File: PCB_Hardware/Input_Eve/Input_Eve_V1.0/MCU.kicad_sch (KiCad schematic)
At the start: 15 parts, among them J1 Conn_ARM_JTAG_SWD_10, U1 STM32H743VITx

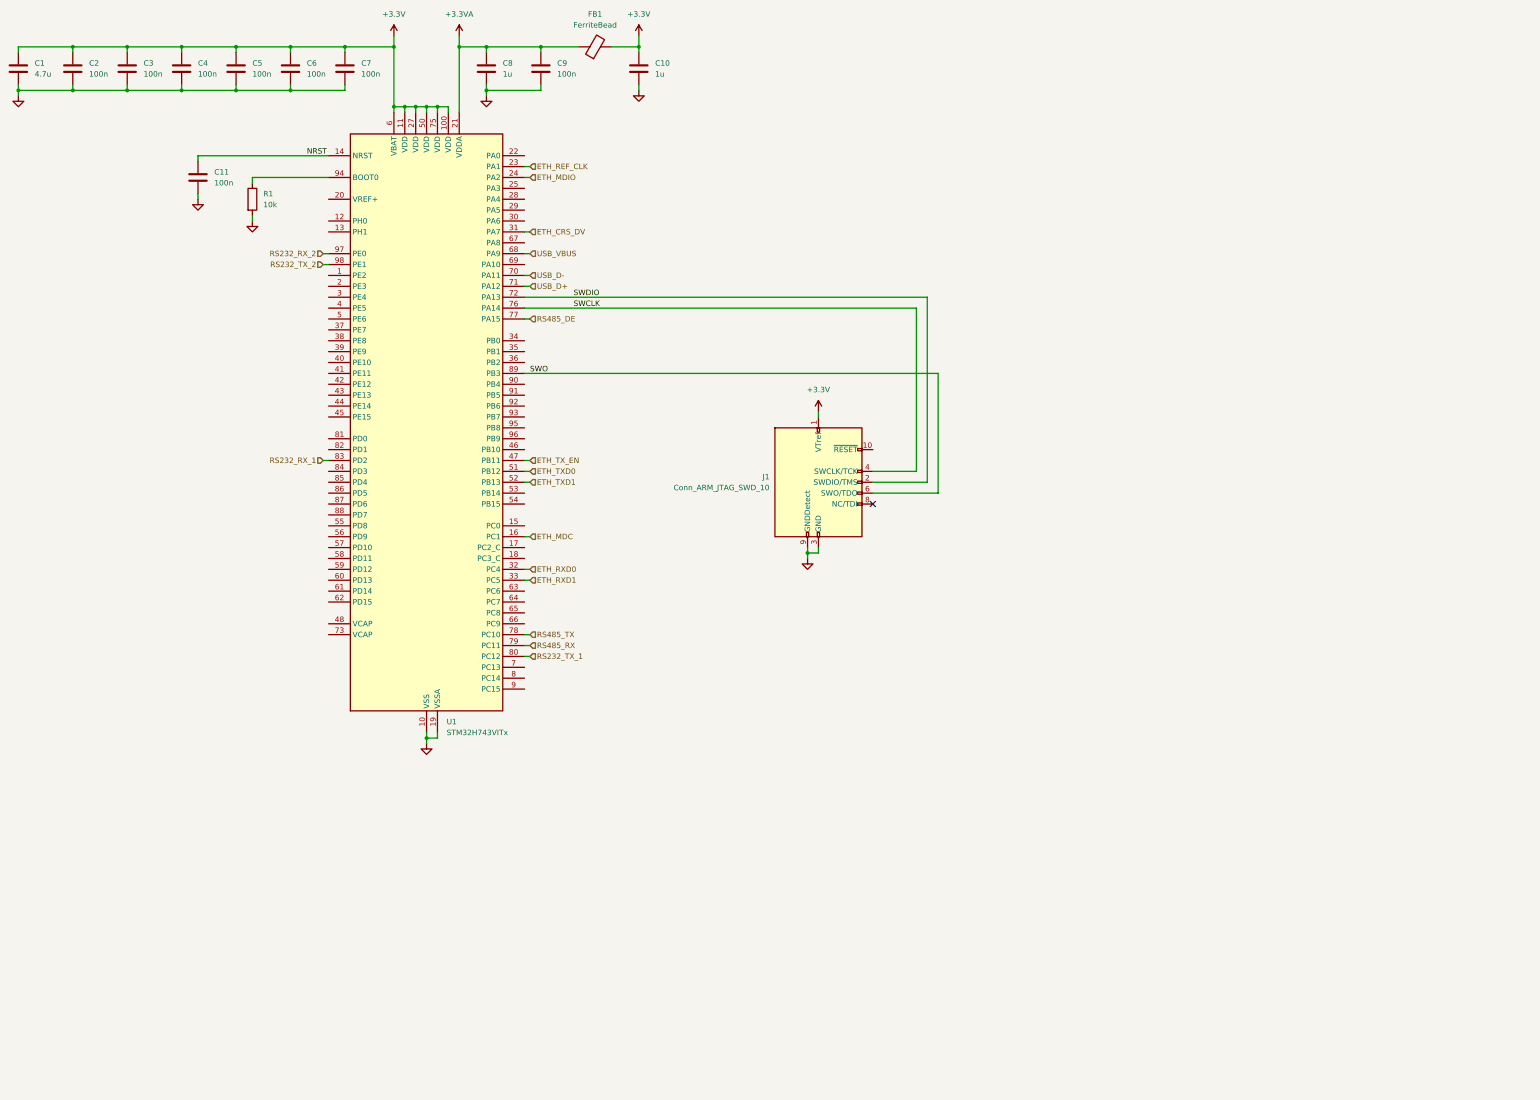
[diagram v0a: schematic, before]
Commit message: Update w new boards/firmware
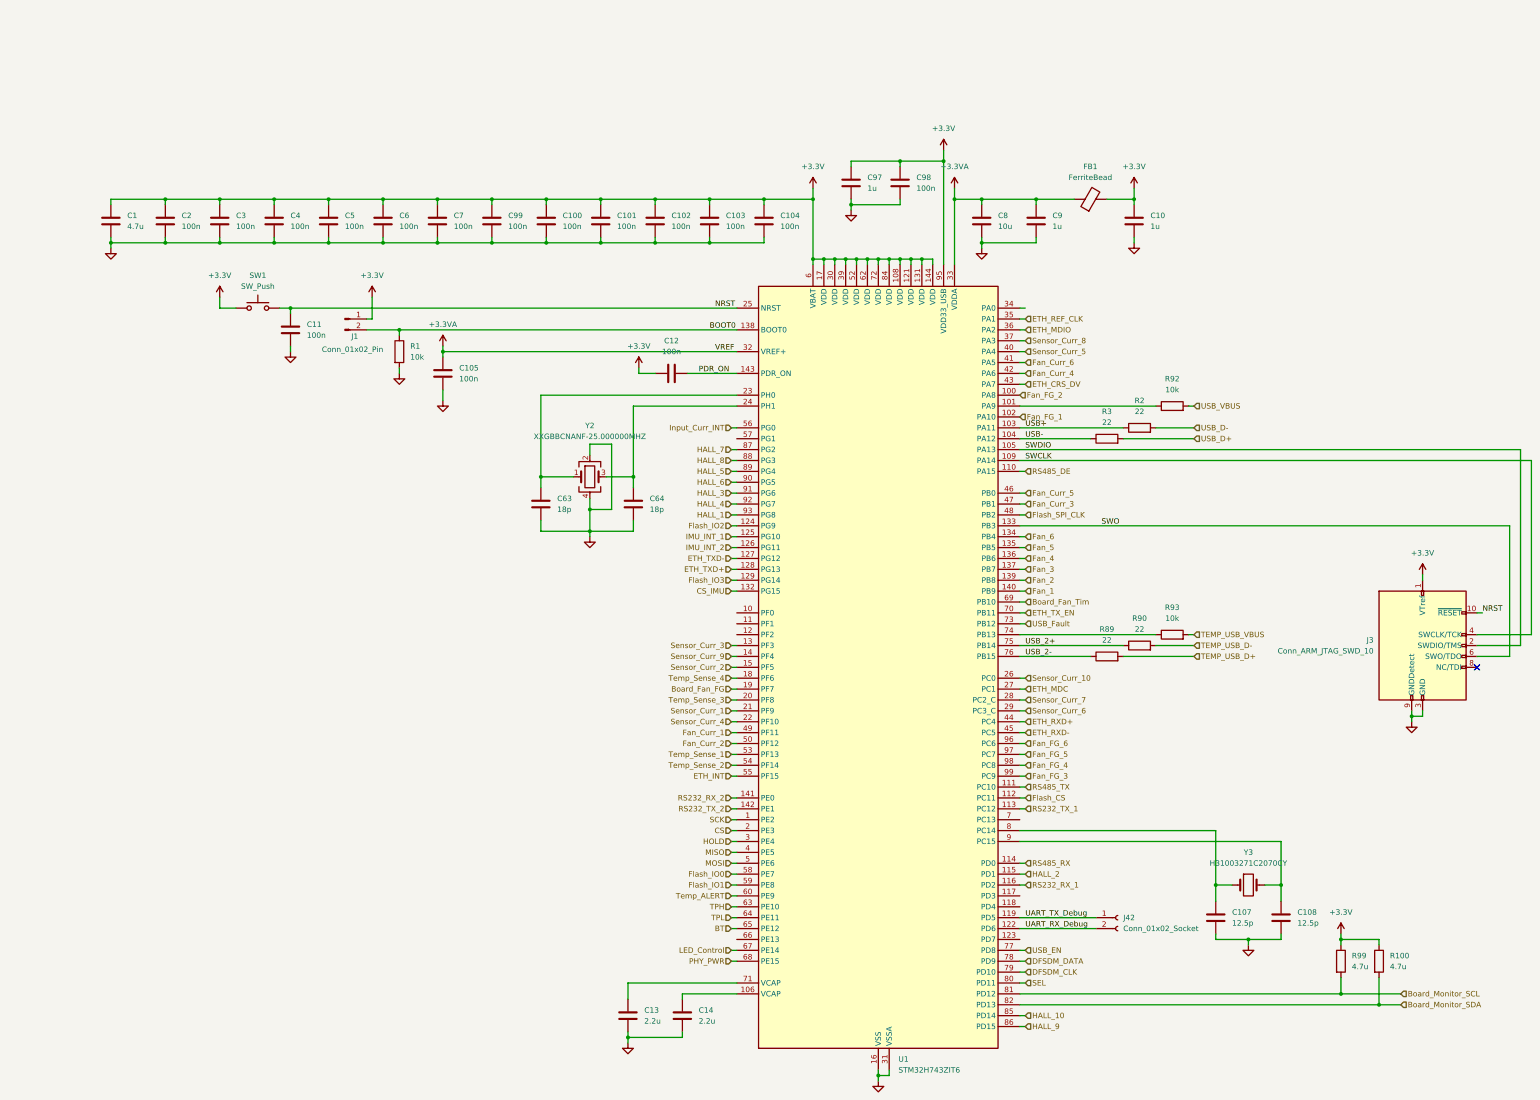
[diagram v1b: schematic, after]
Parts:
- removed U1: STM32H743VITx, Package_QFP:LQFP-100_14x14mm_P0.5mm, symbol MCU_ST_STM32H7:STM32H743VITx
- added C100, C101, C102, C103, C104, C105, C12, C98, C99: 100n, Capacitor_SMD:C_0402_1005Metric, symbol Device:C
- added C107, C108: 12.5p, Capacitor_SMD:C_0402_1005Metric, symbol Device:C
- added C13, C14: 2.2u, Capacitor_SMD:C_0402_1005Metric, symbol Device:C
- added C63, C64: 18p, Capacitor_SMD:C_0402_1005Metric, symbol Device:C
- added C97: 1u, Capacitor_SMD:C_0402_1005Metric, symbol Device:C
- added J1: Conn_01x02_Pin, Connector_PinHeader_2.54mm:PinHeader_1x02_P2.54mm_Vertical, symbol Connector:Conn_01x02_Pin
- added J42: Conn_01x02_Socket, Connector_JST:JST_PH_B2B-PH-K_1x02_P2.00mm_Vertical, symbol Connector:Conn_01x02_Socket
- added R100, R99: 4.7u, Resistor_SMD:R_0402_1005Metric, symbol Device:R
- added R2, R3, R89, R90: 22, Resistor_SMD:R_0402_1005Metric, symbol Device:R
- added R92, R93: 10k, Resistor_SMD:R_0402_1005Metric, symbol Device:R
- added SW1: SW_Push, Tutor_Common_Parts:TSB008A2518A, symbol Switch:SW_Push
- added U1: STM32H743ZIT6, Package_QFP:LQFP-144_20x20mm_P0.5mm, symbol MCU_ST_STM32H7:STM32H743ZITx
- added Y2: XXGBBCNANF-25.000000MHZ, Crystal:Crystal_SMD_3225-4Pin_3.2x2.5mm, symbol Device:Crystal_GND24
- added Y3: H31003271C2070CY, Crystal:Crystal_SMD_3215-2Pin_3.2x1.5mm, symbol Device:Crystal
- C1: footprint (none) -> Capacitor_SMD:C_0603_1608Metric
- C10, C11, C2, C3, C4, C5, C6, C7: footprint (none) -> Capacitor_SMD:C_0402_1005Metric
- C8: renamed from C9; value 100n -> 10u; footprint (none) -> Capacitor_SMD:C_0402_1005Metric
- C9: renamed from C8; footprint (none) -> Capacitor_SMD:C_0402_1005Metric
- FB1: footprint (none) -> Inductor_SMD:L_0603_1608Metric
- J3: renamed from J1; footprint (none) -> Connector_PinHeader_1.27mm:PinHeader_2x05_P1.27mm_Vertical_SMD
- R1: footprint (none) -> Resistor_SMD:R_0402_1005Metric
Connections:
- net +3.3V: now also C100.1, C101.1, C102.1, C103.1, C104.1, C12.1, C97.1, C98.1, C99.1, J1.1 (Pin_1), R100.1, R99.1, SW1.1, U1.108 (VDD), U1.121 (VDD), U1.131 (VDD), U1.144 (VDD), U1.17 (VDD), U1.30 (VDD), U1.39 (VDD), U1.52 (VDD), U1.6 (VBAT), U1.62 (VDD), U1.72 (VDD), U1.84 (VDD), U1.95 (VDD33_USB)
- net +3.3VA: now also C105.2, U1.32 (VREF+), U1.33 (VDDA)
- net ETH_CRS_DV: now also U1.43 (PA7)
- net ETH_MDC: now also U1.27 (PC1)
- net ETH_MDIO: now also U1.36 (PA2)
- net ETH_REF_CLK: now also U1.35 (PA1)
- net ETH_TX_EN: now also U1.70 (PB11)
- net GND: now also C100.2, C101.2, C102.2, C103.2, C104.2, C105.1, C107.2, C108.2, C13.2, C14.2, C63.2, C64.2, C97.2, C98.2, C99.2, U1.107 (VSS), U1.120 (VSS), U1.130 (VSS), U1.16 (VSS), U1.31 (VSSA), U1.38 (VSS), U1.51 (VSS), U1.61 (VSS), U1.83 (VSS), U1.94 (VSS), Y2.2, Y2.4
- net NRST: now also J3.10 (~{RESET}), SW1.2, U1.25 (NRST)
- net RS232_RX_1: now also U1.116 (PD2)
- net RS232_RX_2: now also U1.141 (PE0)
- net RS232_TX_1: now also U1.113 (PC12)
- net RS232_TX_2: now also U1.142 (PE1)
- net RS485_DE: now also U1.110 (PA15)
- net RS485_RX: now also U1.114 (PD0)
- net RS485_TX: now also U1.111 (PC10)
- net SWCLK: now also U1.109 (PA14)
- net SWDIO: now also U1.105 (PA13)
- net SWO: now also U1.133 (PB3)
- net USB_D+: now also R3.2
- net USB_D-: now also R2.2
- net USB_VBUS: now also R92.2
- net BOOT0: now reaches R1.1
- net BOOT0: now also J1.2 (Pin_2), U1.138 (BOOT0)
- new net: C14.1, U1.106 (VCAP)
- new net: C63.1, U1.23 (PH0), Y2.1
- new net: C64.1, U1.24 (PH1), Y2.3
- new net: C107.1, U1.8 (PC14), Y3.1
- new net: C13.1, U1.71 (VCAP)
- new net: R93.1, U1.74 (PB13)
- new net: R92.1, U1.101 (PA9)
- new net: C108.1, U1.9 (PC15), Y3.2
- new net BT: U1.65 (PE12)
- new net Board_Fan_FG: U1.19 (PF7)
- new net Board_Fan_Tim: U1.69 (PB10)
- new net Board_Monitor_SCL: R99.2, U1.81 (PD12)
- new net Board_Monitor_SDA: R100.2, U1.82 (PD13)
- new net CS: U1.2 (PE3)
- new net CS_IMU: U1.132 (PG15)
- new net DFSDM_CLK: U1.79 (PD10)
- new net DFSDM_DATA: U1.78 (PD9)
- new net ETH_INT: U1.55 (PF15)
- new net ETH_RXD+: U1.44 (PC4)
- new net ETH_RXD-: U1.45 (PC5)
- new net ETH_TXD+: U1.128 (PG13)
- new net ETH_TXD-: U1.127 (PG12)
- new net Fan_1: U1.140 (PB9)
- new net Fan_2: U1.139 (PB8)
- new net Fan_3: U1.137 (PB7)
- new net Fan_4: U1.136 (PB6)
- new net Fan_5: U1.135 (PB5)
- new net Fan_6: U1.134 (PB4)
- new net Fan_Curr_1: U1.49 (PF11)
- new net Fan_Curr_2: U1.50 (PF12)
- new net Fan_Curr_3: U1.47 (PB1)
- new net Fan_Curr_4: U1.42 (PA6)
- new net Fan_Curr_5: U1.46 (PB0)
- new net Fan_Curr_6: U1.41 (PA5)
- new net Fan_FG_1: U1.102 (PA10)
- new net Fan_FG_2: U1.100 (PA8)
- new net Fan_FG_3: U1.99 (PC9)
- new net Fan_FG_4: U1.98 (PC8)
- new net Fan_FG_5: U1.97 (PC7)
- new net Fan_FG_6: U1.96 (PC6)
- new net Flash_CS: U1.112 (PC11)
- new net Flash_IO0: U1.58 (PE7)
- new net Flash_IO1: U1.59 (PE8)
- new net Flash_IO2: U1.124 (PG9)
- new net Flash_IO3: U1.129 (PG14)
- new net Flash_SPI_CLK: U1.48 (PB2)
- new net HALL_1: U1.93 (PG8)
- new net HALL_10: U1.85 (PD14)
- new net HALL_2: U1.115 (PD1)
- new net HALL_3: U1.91 (PG6)
- new net HALL_4: U1.92 (PG7)
- new net HALL_5: U1.89 (PG4)
- new net HALL_6: U1.90 (PG5)
- new net HALL_7: U1.87 (PG2)
- new net HALL_8: U1.88 (PG3)
- new net HALL_9: U1.86 (PD15)
- new net HOLD: U1.3 (PE4)
- new net IMU_INT_1: U1.125 (PG10)
- new net IMU_INT_2: U1.126 (PG11)
- new net Input_Curr_INT: U1.56 (PG0)
- new net LED_Control: U1.67 (PE14)
- new net MISO: U1.4 (PE5)
- new net MOSI: U1.5 (PE6)
- new net PDR_ON: C12.2, U1.143 (PDR_ON)
- new net PHY_PWR: U1.68 (PE15)
- new net SCK: U1.1 (PE2)
- new net SEL: U1.80 (PD11)
- new net Sensor_Curr_1: U1.21 (PF9)
- new net Sensor_Curr_10: U1.26 (PC0)
- new net Sensor_Curr_2: U1.15 (PF5)
- new net Sensor_Curr_3: U1.13 (PF3)
- new net Sensor_Curr_4: U1.22 (PF10)
- new net Sensor_Curr_5: U1.40 (PA4)
- new net Sensor_Curr_6: U1.29 (PC3_C)
- new net Sensor_Curr_7: U1.28 (PC2_C)
- new net Sensor_Curr_8: U1.37 (PA3)
- new net Sensor_Curr_9: U1.14 (PF4)
- new net TEMP_USB_D+: R89.2
- new net TEMP_USB_D-: R90.2
- new net TEMP_USB_VBUS: R93.2
- new net TPH: U1.63 (PE10)
- new net TPL: U1.64 (PE11)
- new net Temp_ALERT: U1.60 (PE9)
- new net Temp_Sense_1: U1.53 (PF13)
- new net Temp_Sense_2: U1.54 (PF14)
- new net Temp_Sense_3: U1.20 (PF8)
- new net Temp_Sense_4: U1.18 (PF6)
- new net UART_RX_Debug: J42.2 (Pin_2), U1.122 (PD6)
- new net UART_TX_Debug: J42.1 (Pin_1), U1.119 (PD5)
- new net USB+: R2.1, U1.103 (PA11)
- new net USB-: R3.1, U1.104 (PA12)
- new net USB_2+: R90.1, U1.75 (PB14)
- new net USB_2-: R89.1, U1.76 (PB15)
- new net USB_EN: U1.77 (PD8)
- new net USB_Fault: U1.73 (PB12)
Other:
- moved on the sheet: C1, C10, C11, C2, C3, C4, C5, C6, C7, C8, C9, FB1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
